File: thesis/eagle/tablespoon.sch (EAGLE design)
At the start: 26 parts, among them IC1 7805DT, IC2 7805DT, U1 ADCS7477

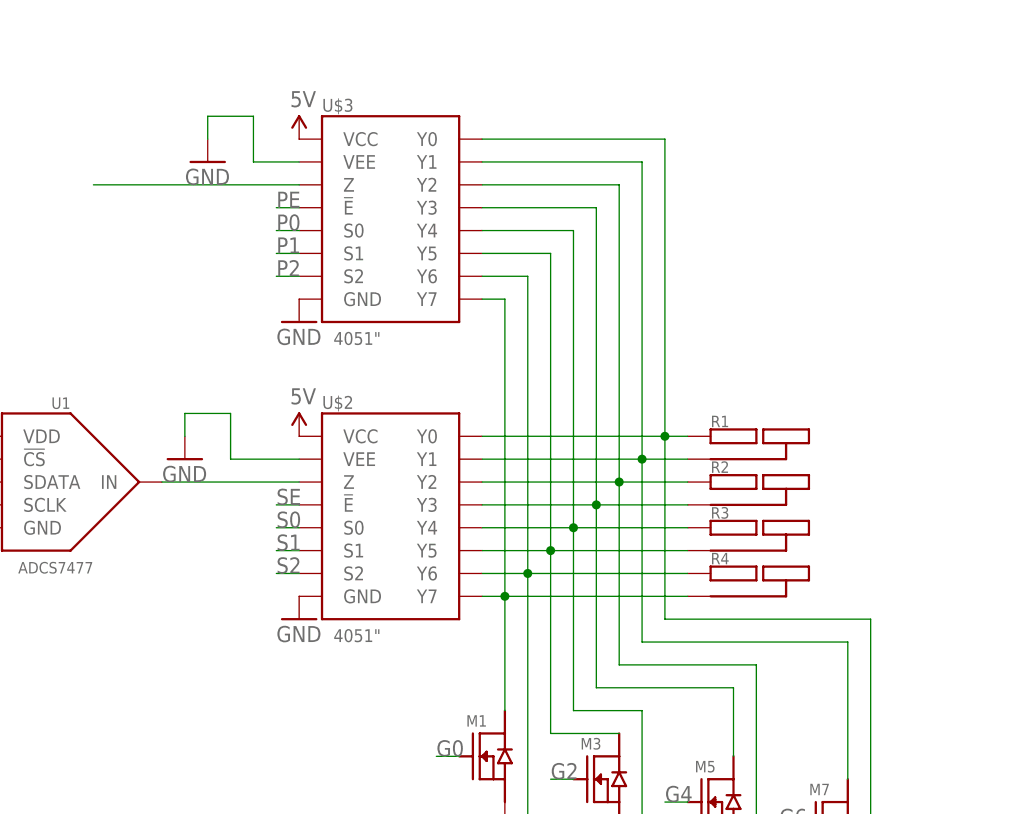
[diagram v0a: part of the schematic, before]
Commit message: oh when you're done with that teaspoon, do i gotta tablespoon fer you!
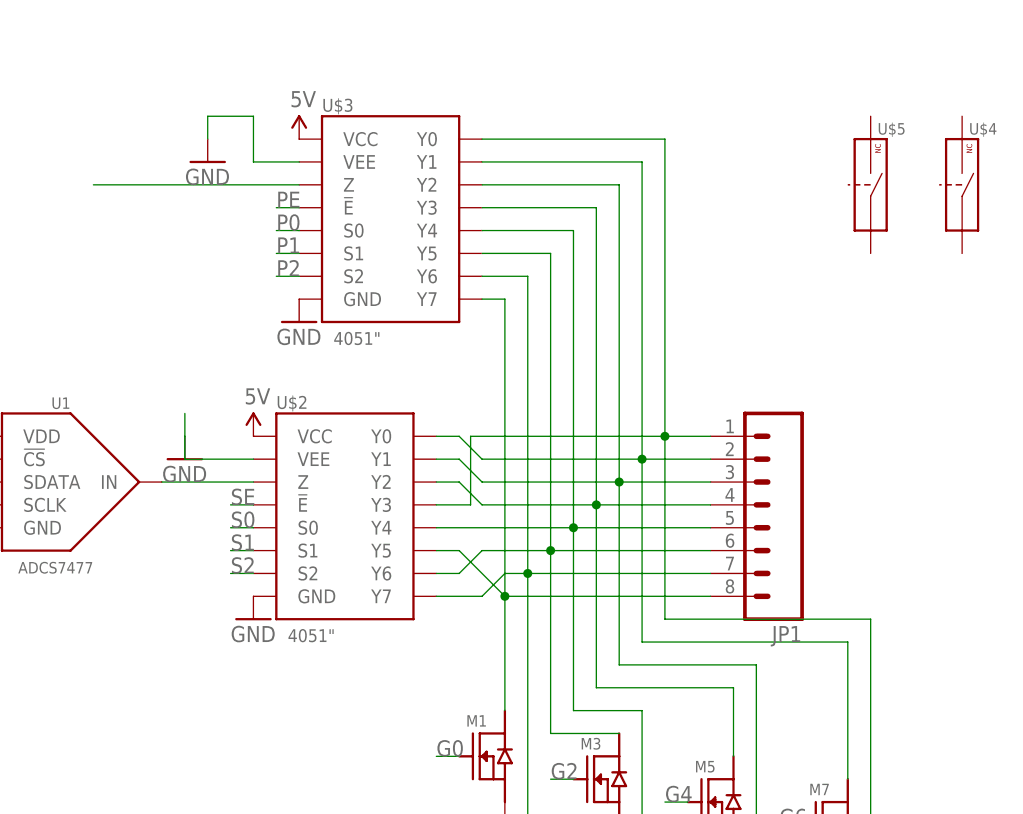
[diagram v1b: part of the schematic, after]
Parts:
- removed R1, R2, R3, R4: RAILROW, butter:RAILROW
- added JP1: (no value), SparkFun-Connectors:M08LONGPADS
- added U$4, U$5: DG467, butter:DG467
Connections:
- net N$10: now also JP1.3, U$2.Y1; no longer R2.L, U$2.Y2
- net N$11: now also JP1.4, U$2.Y2; no longer R2.R, U$2.Y3
- net N$12: now also JP1.5; no longer R3.L
- net N$13: now also JP1.6, U$2.Y6; no longer R3.R, U$2.Y5
- net N$14: now also JP1.7, U$2.Y7; no longer R4.L, U$2.Y6
- net N$15: now also JP1.8, U$2.Y5; no longer R4.R
- net N$8: now also JP1.1, U$2.Y3; no longer R1.L, U$2.Y0
- net N$9: now also JP1.2, U$2.Y0; no longer R1.R, U$2.Y1
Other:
- moved on the sheet: U$2
